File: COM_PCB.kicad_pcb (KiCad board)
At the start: 2 copper layers, 70 x 70 mm, 55 parts, among them J1 Conn_Coaxial, J2 SIM_Card, J3 ST_LINK, J4 Conn_Coaxial, J6 02x12, SW1 Reset, U1 STM32F401CEUx, U2 NEO-6M-0-001, U3 Ai-Thinker_Ra-02, Y1 MCSJK

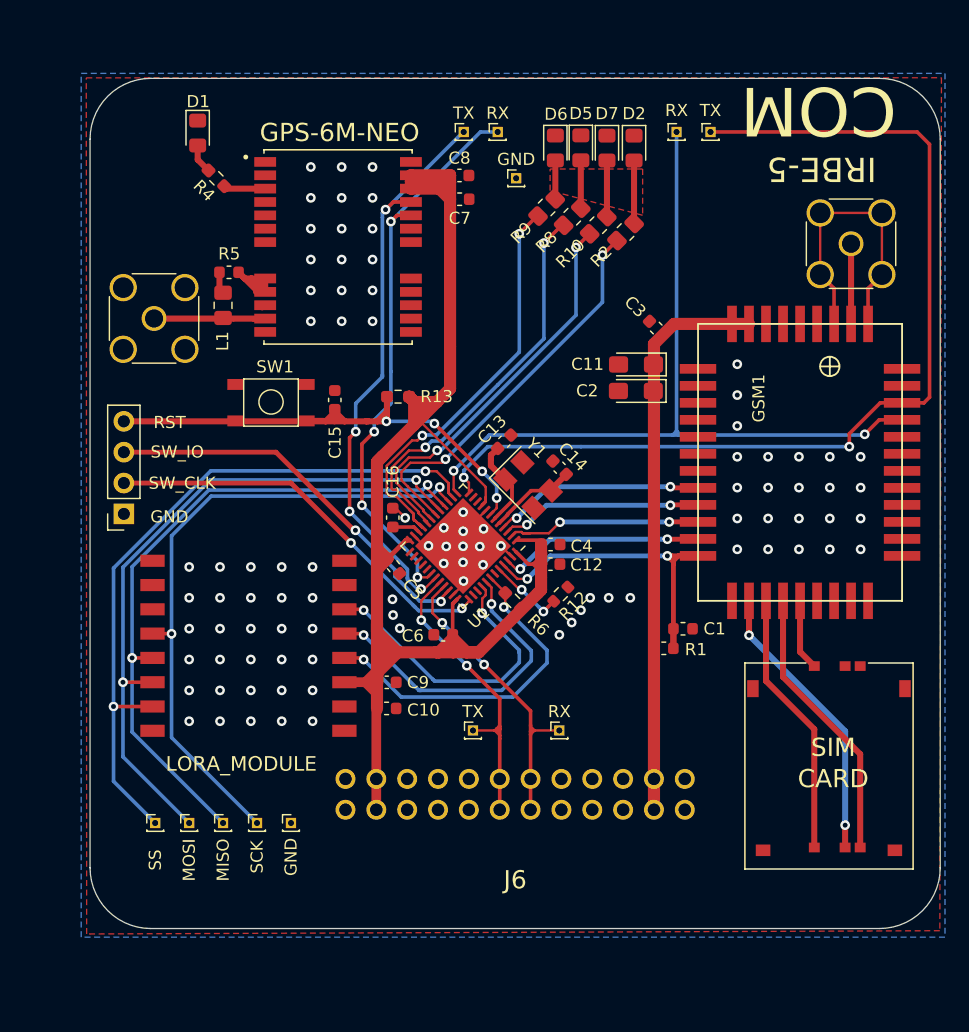
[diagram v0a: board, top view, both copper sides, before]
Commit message: KiCad 0.3v
Improved aesthetics.
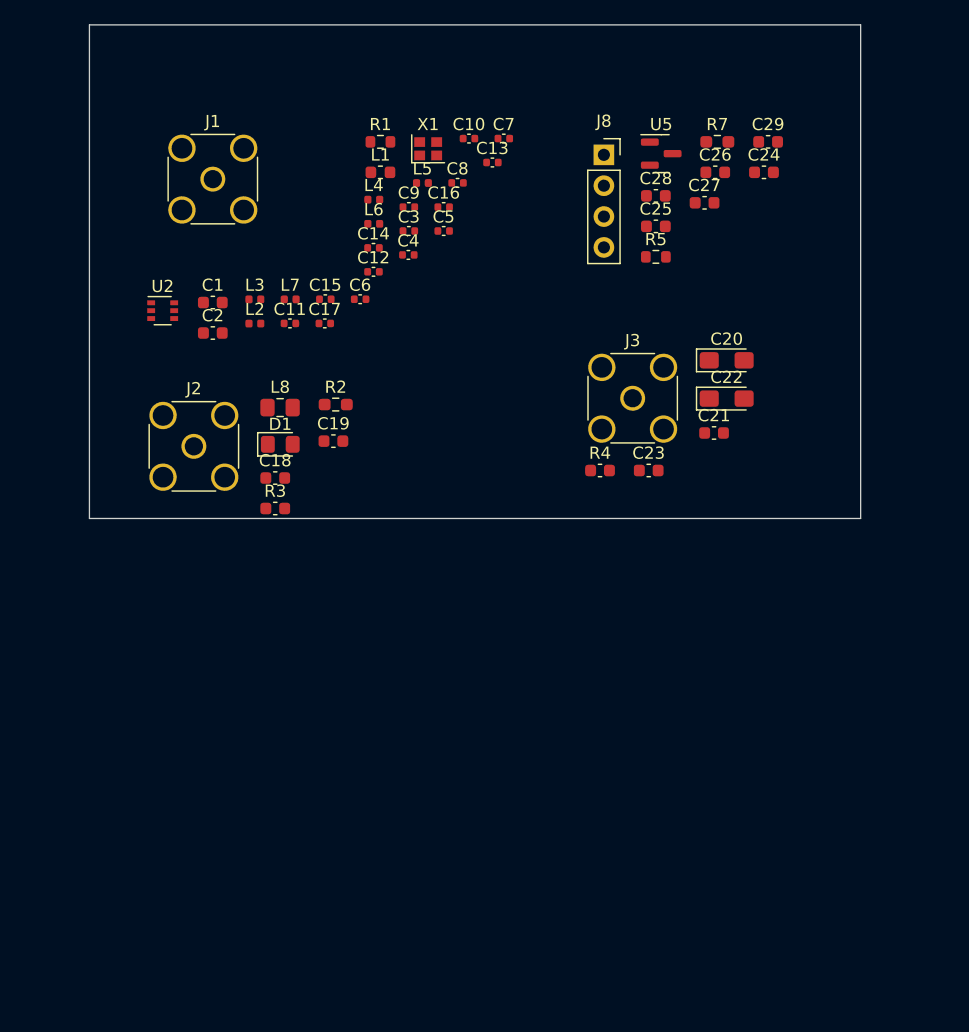
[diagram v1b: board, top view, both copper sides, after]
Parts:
- removed D2, D5, D6, D7: BLUE, LED_SMD:LED_0805_2012Metric_Pad1.15x1.40mm_HandSolder
- removed GND (x2), MISO, MOSI, RX (x3), SCK, SS, TX (x3): TestPoint, Connector_PinHeader_1.00mm:PinHeader_1x01_P1.00mm_Vertical
- removed GSM1: A6_GSM, A6:A6_GSM
- removed J4: Conn_Coaxial, Connector_Coaxial:SMA_Amphenol_132134-16_Vertical
- removed J6: 02x12, LOCAL:SAMTEC-SSW-112-02-X-D-RA
- removed R10, R8, R9: 75, Resistor_SMD:R_0805_2012Metric_Pad1.20x1.40mm_HandSolder
- removed R12: 12k, Resistor_SMD:R_0603_1608Metric
- removed R13: 12k, Resistor_SMD:R_0603_1608Metric_Pad0.98x0.95mm_HandSolder
- removed R6: 10k, Resistor_SMD:R_0603_1608Metric_Pad0.98x0.95mm_HandSolder
- removed SW1: Reset, button:little_button
- removed U1: STM32F401CEUx, Package_DFN_QFN:QFN-48-1EP_7x7mm_P0.5mm_EP5.6x5.6mm
- removed U3: Ai-Thinker_Ra-02, LOCAL:Ai-Thinker_Ra-02
- removed Y1: MCSJK, Crystal:Crystal_SMD_5032-4Pin_5.0x3.2mm
- added C17: 2.4pF, Capacitor_SMD:C_0402_1005Metric, F.Cu at (115.9, 77.9)
- added C18: 0.1uF, Capacitor_SMD:C_0603_1608Metric, F.Cu at (111.8, 90.7)
- added C19: 10uF, Capacitor_SMD:C_0603_1608Metric, F.Cu at (116.6, 87.6)
- added C20: 220uF, Capacitor_Tantalum_SMD:CP_EIA-3216-10_Kemet-I_Pad1.58x1.35mm_HandSolder, F.Cu at (149.0, 81.0)
- added C21: 0.1uF, Capacitor_SMD:C_0603_1608Metric, F.Cu at (147.9, 86.9)
- added C22: 220uF, Capacitor_Tantalum_SMD:CP_EIA-3216-10_Kemet-I_Pad1.58x1.35mm_HandSolder, F.Cu at (149.0, 84.1)
- added C23: 0.1uF, Capacitor_SMD:C_0603_1608Metric, F.Cu at (142.6, 90.0)
- added C24: 0.1uF, Capacitor_SMD:C_0603_1608Metric, F.Cu at (152.1, 65.5)
- added C25: 0.1uF, Capacitor_SMD:C_0603_1608Metric, F.Cu at (143.2, 69.9)
- added C26: 0.1uF, Capacitor_SMD:C_0603_1608Metric, F.Cu at (148.1, 65.5)
- added C27: 12.5pF, Capacitor_SMD:C_0603_1608Metric, F.Cu at (147.2, 68.0)
- added C28: 220nF, Capacitor_SMD:C_0603_1608Metric, F.Cu at (143.2, 67.4)
- added C29: 12.5pF, Capacitor_SMD:C_0603_1608Metric, F.Cu at (152.4, 63.0)
- added J8: ST_LINK, Connector_PinSocket_2.54mm:PinSocket_1x04_P2.54mm_Vertical, F.Cu at (138.9, 64.0)
- added L2: 33nH, Inductor_SMD:L_0402_1005Metric, F.Cu at (110.1, 77.9)
- added L3: 30nH, Inductor_SMD:L_0402_1005Metric, F.Cu at (110.1, 75.9)
- added L4: 36nH, Inductor_SMD:L_0402_1005Metric, F.Cu at (119.9, 67.7)
- added L5: 22nH, Inductor_SMD:L_0402_1005Metric, F.Cu at (123.9, 66.4)
- added L6: 62nH, Inductor_SMD:L_0402_1005Metric, F.Cu at (119.9, 69.7)
- added L7: 56nH, Inductor_SMD:L_0402_1005Metric, F.Cu at (113.0, 75.9)
- added L8: 27uH, Capacitor_SMD:C_0805_2012Metric_Pad1.18x1.45mm_HandSolder, F.Cu at (112.2, 84.8)
- added R3: 10, Capacitor_SMD:C_0603_1608Metric, F.Cu at (111.8, 93.2)
- added R7: 12k, Resistor_SMD:R_0603_1608Metric_Pad0.98x0.95mm_HandSolder, F.Cu at (148.2, 63.0)
- added U5: LM4040DBZ-3, Package_TO_SOT_SMD:SOT-23, F.Cu at (143.6, 63.9)
- added X1: TCXO 26 MHz, Crystal:Crystal_SMD_2016-4Pin_2.0x1.6mm, F.Cu at (124.4, 63.5)
- C1: value 0.1uF -> 4.7uF
- C10: value 0.1uF -> 100pF; footprint Capacitor_SMD:C_0603_1608Metric -> Capacitor_SMD:C_0402_1005Metric
- C11: value 220uF -> 10pF; footprint Capacitor_Tantalum_SMD:CP_EIA-3216-10_Kemet-I_Pad1.58x1.35mm_HandSolder -> Capacitor_SMD:C_0402_1005Metric
- C12: value 0.1uF -> 680pF; footprint Capacitor_SMD:C_0603_1608Metric -> Capacitor_SMD:C_0402_1005Metric
- C13: value 22pF -> 680pF; footprint Capacitor_SMD:C_0603_1608Metric -> Capacitor_SMD:C_0402_1005Metric
- C14: value 22pF -> 10pF; footprint Capacitor_SMD:C_0603_1608Metric -> Capacitor_SMD:C_0402_1005Metric
- C15: value 220nF -> 680pF; footprint Capacitor_SMD:C_0603_1608Metric -> Capacitor_SMD:C_0402_1005Metric
- C16: value 4.7uF -> 4.7pF; footprint Capacitor_SMD:C_0603_1608Metric -> Capacitor_SMD:C_0402_1005Metric
- C2: value 220uF -> 4.7uF; footprint Capacitor_Tantalum_SMD:CP_EIA-3216-10_Kemet-I_Pad1.58x1.35mm_HandSolder -> Capacitor_SMD:C_0603_1608Metric
- C3, C4, C5: footprint Capacitor_SMD:C_0603_1608Metric -> Capacitor_SMD:C_0402_1005Metric
- C6: value 0.1uF -> 9.1pF; footprint Capacitor_SMD:C_0603_1608Metric -> Capacitor_SMD:C_0402_1005Metric
- C7: value 0.1uF -> 15pF; footprint Capacitor_SMD:C_0603_1608Metric -> Capacitor_SMD:C_0402_1005Metric
- C8: value 10uF -> 10nF; footprint Capacitor_SMD:C_0603_1608Metric -> Capacitor_SMD:C_0402_1005Metric
- C9: value 10uF -> 12pF; footprint Capacitor_SMD:C_0603_1608Metric -> Capacitor_SMD:C_0402_1005Metric
- J1: value Conn_Coaxial -> SMA
- J2: value SIM_Card -> SMA; footprint footprints:MOLEX_78800-0001 -> Connector_Coaxial:SMA_Amphenol_132134-16_Vertical
- J3: value ST_LINK -> SMA; footprint Connector_PinSocket_2.54mm:PinSocket_1x04_P2.54mm_Vertical -> Connector_Coaxial:SMA_Amphenol_132134-16_Vertical
- L1: value 27uH -> 220nH; footprint Capacitor_SMD:C_0805_2012Metric_Pad1.18x1.45mm_HandSolder -> Inductor_SMD:L_0603_1608Metric
- R1: value 10k -> 24; footprint Capacitor_SMD:C_0603_1608Metric -> Resistor_SMD:R_0603_1608Metric
- R2: value 75 -> 1k; footprint Resistor_SMD:R_0805_2012Metric_Pad1.20x1.40mm_HandSolder -> Resistor_SMD:R_0603_1608Metric_Pad0.98x0.95mm_HandSolder
- R4: value 1k -> 10k; footprint Resistor_SMD:R_0603_1608Metric_Pad0.98x0.95mm_HandSolder -> Capacitor_SMD:C_0603_1608Metric
- R5: value 10 -> 12k; footprint Capacitor_SMD:C_0603_1608Metric -> Resistor_SMD:R_0603_1608Metric
- U2: value NEO-6M-0-001 -> AS179-92LF; footprint footprints:XCVR_NEO-6M-GPS -> Package_TO_SOT_SMD:SOT-363_SC-70-6
- moved J2 58.5 mm to (105.1, 88.0), turned to 0 degrees
- moved J1 52.8 mm to (106.7, 66.0), turned to 0 degrees
- moved R1 47.8 mm to (120.5, 63.0)
- moved C10 47.4 mm to (127.8, 62.7)
- moved C1 47.1 mm to (106.7, 76.2)
- moved J3 43.0 mm to (141.2, 84.1), turned to 0 degrees
- moved R4 39.7 mm to (138.6, 90.0), turned to 0 degrees
- moved C9 39.2 mm to (122.8, 68.3)
- moved R5 35.2 mm to (143.2, 72.4), turned to 0 degrees
- moved C2 35.2 mm to (106.7, 78.7), turned to 0 degrees
- moved C11 28.7 mm to (113.0, 77.9), turned to 0 degrees
- moved C6 28.5 mm to (118.8, 75.9), turned to 0 degrees
- moved C12 28.1 mm to (119.9, 73.7)
- moved C5 27.9 mm to (125.7, 70.3), turned to 0 degrees
- moved R2 27.8 mm to (116.8, 84.6), turned to 0 degrees
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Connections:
- C1 pad 1: (no net) -> +3V3
- C1 pad 2: (no net) -> GND
- C10 pad 1: (no net) -> Net-(C10-Pad1)
- C10 pad 2: (no net) -> /SI4463/XOUT
- C11 pad 1: (no net) -> GND
- C11 pad 2: (no net) -> Net-(C11-Pad2)
- C12 pad 1: (no net) -> Net-(C12-Pad1)
- C12 pad 2: (no net) -> /SI4463/TX
- C13 pad 1: (no net) -> /SI4463/RX
- C13 pad 2: (no net) -> Net-(C13-Pad2)
- C14 pad 1: (no net) -> /SI4463/TX
- C14 pad 2: (no net) -> /SI4463/TX_F
- C15 pad 1: (no net) -> Net-(C15-Pad1)
- C15 pad 2: (no net) -> /SI4463/ANT
- C16 pad 1: (no net) -> GND
- C16 pad 2: (no net) -> /SI4463/RXp
- C2 pad 1: (no net) -> +3V3
- C2 pad 2: (no net) -> GND
- C3 pad 1: (no net) -> +3V3
- C3 pad 2: (no net) -> GND
- C4 pad 1: (no net) -> +3V3
- C4 pad 2: (no net) -> GND
- C5 pad 1: (no net) -> GND
- C5 pad 2: (no net) -> +3V3
- C6 pad 1: (no net) -> Net-(C6-Pad1)
- C6 pad 2: (no net) -> /SI4463/TX_UM
- C7 pad 1: (no net) -> GND
- C7 pad 2: (no net) -> /SI4463/TX_M
- C8 pad 1: (no net) -> GND
- C8 pad 2: (no net) -> +3V3
- C9 pad 1: (no net) -> GND
- C9 pad 2: (no net) -> Net-(C9-Pad2)
- D1 pad 1: (no net) -> GND
- D1 pad 2: (no net) -> Net-(D1-Pad2)
- J1 pad 1: (no net) -> /SI4463/ANT
- J1 pad 2: (no net) -> GND
- J2 pad 1: (no net) -> /GPS/ANT
- J2 pad 2: (no net) -> GND
- J3 pad 1: (no net) -> /GPRS/ANT
- J3 pad 2: (no net) -> GND
- L1 pad 1: (no net) -> /SI4463/TX_UM
- L1 pad 2: (no net) -> Net-(L1-Pad2)
- R1 pad 1: (no net) -> +3V3
- R1 pad 2: (no net) -> Net-(L1-Pad2)
- R2 pad 1: (no net) -> Net-(R2-Pad1)
- R2 pad 2: (no net) -> Net-(D1-Pad2)
- R4 pad 1: (no net) -> +4V
- R4 pad 2: (no net) -> /GPRS/GSM_RST
- R5 pad 1: (no net) -> /MCU/SW_CLK
- R5 pad 2: (no net) -> GND
- U2 pad 1: (no net) -> Net-(C12-Pad1)
- U2 pad 2: (no net) -> GND
- U2 pad 3: (no net) -> Net-(C13-Pad2)
- U2 pad 4: (no net) -> /SI4463/GPIO2
- U2 pad 5: (no net) -> Net-(C15-Pad1)
- U2 pad 6: (no net) -> /SI4463/GPIO3
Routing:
- net (no net): track 1353.2 -> 0.00 mm, vias 154 -> 0
- removed copper zone on B.Cu, net (none)
- removed copper zone on F.Cu, net (none)
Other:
- board size 70 x 70 mm -> 63.5 x 40.6 mm
- board text removed: "CARD"
- board text removed: "COM"
- board text removed: "GND"
- board text removed: "GPS-6M-NEO"
- board text removed: "IRBE-5"
- board text removed: "LORA_MODULE"
- board text removed: "Physical connector"
- board text removed: "RST"
- board text removed: "SIM"
- board text removed: "SW_CLK"
- board text removed: "SW_IO"

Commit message: 0.1v COM_PCB KiCad
First iteration of COM PCB.
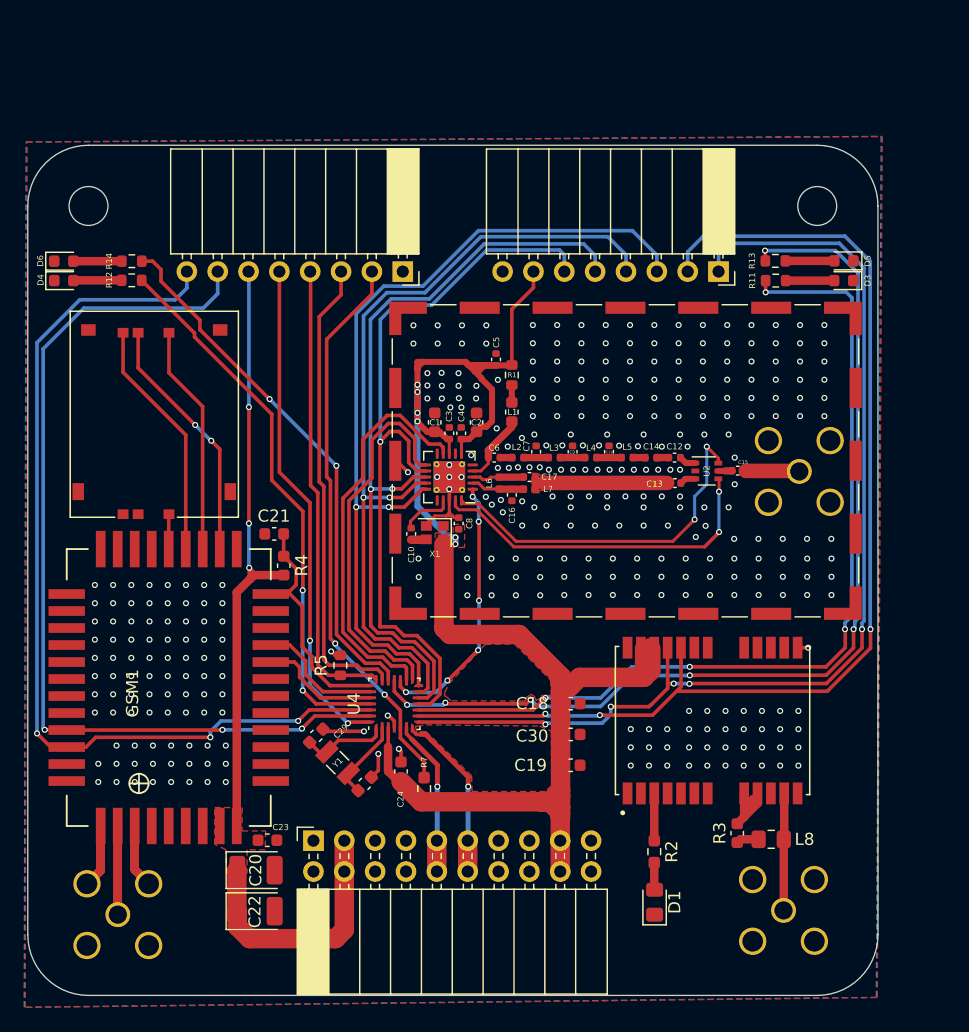
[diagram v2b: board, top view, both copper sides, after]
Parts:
- removed C25, C26: 0.1uF, Capacitor_SMD:C_0603_1608Metric
- removed C28: 220nF, Capacitor_SMD:C_0603_1608Metric
- removed U5: LM4040DBZ-3, Package_TO_SOT_SMD:SOT-23
- added C30: 4.7uF, Capacitor_SMD:C_0603_1608Metric, F.Cu at (136.1, 111.8)
- added D3: LED, LED_SMD:LED_0603_1608Metric, F.Cu at (158.6, 74.4)
- added D4: LED, LED_SMD:LED_0603_1608Metric, F.Cu at (94.4, 74.4)
- added D5: LED, LED_SMD:LED_0603_1608Metric, F.Cu at (158.6, 72.8)
- added D6: LED, LED_SMD:LED_0603_1608Metric, F.Cu at (94.4, 72.8)
- added GSM1: A6_GSM, footprints:A6_GSM, F.Cu at (103.0, 107.9)
- added H1: Spacer, MountingHole:MountingHole_3.2mm_M3, F.Cu at (96.4, 68.2)
- added H2: Spacer, MountingHole:MountingHole_3.2mm_M3, F.Cu at (156.4, 68.2)
- added J4: Card_Holder, footprints:MOLEX_78800-0001, F.Cu at (101.9, 85.4)
- added J5: BackBone, Connector_PinSocket_2.54mm:PinSocket_2x10_P2.54mm_Horizontal, F.Cu at (115.0, 120.5)
- added J6: D1, Connector_PinSocket_2.54mm:PinSocket_1x08_P2.54mm_Horizontal, F.Cu at (122.3, 73.7)
- added J7: D2, Connector_PinSocket_2.54mm:PinSocket_1x08_P2.54mm_Horizontal, F.Cu at (148.3, 73.7)
- added R11: 120, Resistor_SMD:R_0603_1608Metric, F.Cu at (153.0, 74.4)
- added R12: 120, Resistor_SMD:R_0603_1608Metric, F.Cu at (100.0, 74.4)
- added R13: 120, Resistor_SMD:R_0603_1608Metric, F.Cu at (153.0, 72.8)
- added R14: 120, Resistor_SMD:R_0603_1608Metric, F.Cu at (100.0, 72.8)
- added U1: SI4463, Package_DFN_QFN:QFN-20-1EP_4x4mm_P0.5mm_EP2.6x2.6mm_ThermalVias, F.Cu at (126.2, 90.6)
- added U3: NEO-6M-0-001, footprints:XCVR_NEO-6M-GPS, F.Cu at (147.8, 110.6)
- added U4: STM32G071GBU, Package_DFN_QFN:QFN-28_4x4mm_P0.5mm, F.Cu at (121.6, 109.2)
- added Y1: FC-135R_32.7680KA-AG0, footprints:XTAL_FC-135R_32.7680KA-AG0, F.Cu at (117.0, 114.1)
- C19: value 10uF -> 4.7uF
- C20, C22: footprint Capacitor_Tantalum_SMD:CP_EIA-3216-10_Kemet-I_Pad1.58x1.35mm_HandSolder -> Capacitor_Tantalum_SMD:CP_EIA-3528-21_Kemet-B
- C8: value 10nF -> 100nF
- J1, J2, J3: moved to B.Cu
- J8: value ST_LINK -> BMI-S-205-C; footprint Connector_PinSocket_2.54mm:PinSocket_1x04_P2.54mm_Vertical -> RF_Shielding:Laird_Technologies_BMI-S-205-F_38.10x25.40mm
- L8: value 27uH -> 30uH
- R2: value 1k -> 12k
- R4: value 10k -> 12k
- X1: value TCXO 26 MHz -> TCXO 30 MHz
- moved J2 61.8 mm to (153.7, 126.2), turned to 90 degrees
- moved C29 61.4 mm to (115.2, 111.9), turned to 45 degrees
- moved J3 60.0 mm to (98.9, 126.6), turned to 180 degrees
- moved R7 58.5 mm to (124.1, 116.2), turned to 90 degrees
- moved C24 57.7 mm to (122.2, 114.8), turned to 90 degrees
- moved C22 57.3 mm to (110.2, 126.3)
- moved C20 57.1 mm to (110.2, 122.9)
- moved C27 55.4 mm to (119.2, 115.8), turned to -135 degrees
- moved J1 54.0 mm to (155.0, 90.1), turned to 180 degrees
- moved L8 53.8 mm to (152.7, 120.4), turned to 180 degrees
- moved D1 48.7 mm to (143.1, 125.6), turned to 90 degrees
- moved U2 46.7 mm to (147.4, 90.1)
- moved R3 46.5 mm to (149.9, 119.9), turned to -90 degrees
- moved R2 45.2 mm to (143.0, 121.4), turned to -90 degrees
- moved C23 43.7 mm to (111.2, 120.5)
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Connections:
- R5 pad 1: /MCU/SW_CLK -> /IO/SW_CLK
- R7 pad 2: /MCU/~{RST} -> /IO/~{RST}
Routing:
- net +3V3: track 0.00 -> 132.5 mm, vias 0 -> 6
- net /GPS/GPS_TX: track 0.00 -> 93.3 mm, vias 0 -> 3
- net /GPS/GPS_RX: track 0.00 -> 88.8 mm, vias 0 -> 5
- net /MCU/LED1: track 0.00 -> 82.7 mm, vias 0 -> 6
- net /GPRS/GSM_RX: track 0.00 -> 77.2 mm, vias 0 -> 3
- net /GPRS/GSM_TX: track 0.00 -> 76.8 mm, vias 0 -> 3
- net /MCU/LED3: track 0.00 -> 74.6 mm, vias 0 -> 4
- net +4V: track 0.00 -> 72.1 mm, vias 0 -> 3
- net /IO/RF_NSS: track 0.00 -> 70.2 mm, vias 0 -> 2
- net /IO/RF_MOSI: track 0.00 -> 67.1 mm, vias 0 -> 2
- net /IO/RF_MISO: track 0.00 -> 63.4 mm, vias 0 -> 2
- net /IO/RF_SCK: track 0.00 -> 62.0 mm, vias 0 -> 1
- net /IO/~{RST}: track 0.00 -> 46.5 mm, vias 0 -> 2
- net /MCU/LED2: track 0.00 -> 45.4 mm, vias 0 -> 2
- net /MCU/LED0: track 0.00 -> 44.2 mm, vias 0 -> 2
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- added copper zone on F.Cu, net (none)
- added copper zone on F.Cu, net +3V3
- added copper zone on F.Cu, net +4V
- added copper zone on B.Cu, net GND
- added copper zone on F.Cu, net GND
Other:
- board size 63.5 x 40.6 mm -> 70 x 70 mm
- board text added: "Physical connector"
